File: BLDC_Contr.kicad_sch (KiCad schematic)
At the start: 100 parts, among them J1 XT60, J10 PH, J2 Conn_ARM_SWD_TagConnect_TC2030, J3 PH, J4 PH, J5 PH, J6 PH, J7 PH, J8 PIN, Q1 CSD18540Q5B, Q2 CSD18540Q5B, Q3 CSD18540Q5B, Q4 CSD18540Q5B, Q5 CSD18540Q5B, Q6 CSD18540Q5B, U1 STM32G431CBU6, U2 DRV8323RSRGZR, U3 AMS1117-3.3, Y1 Crystal_16Mhz

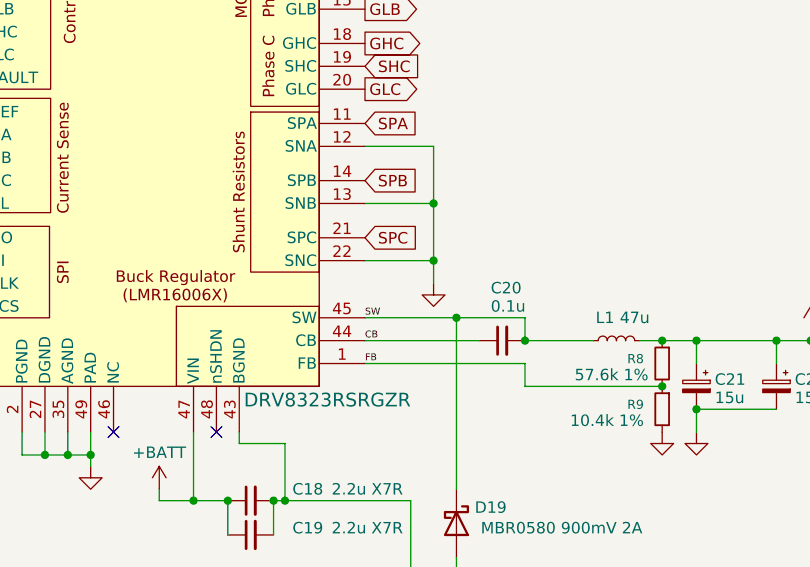
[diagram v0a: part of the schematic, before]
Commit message: wired every component, ground poured doing erc (not done yet)
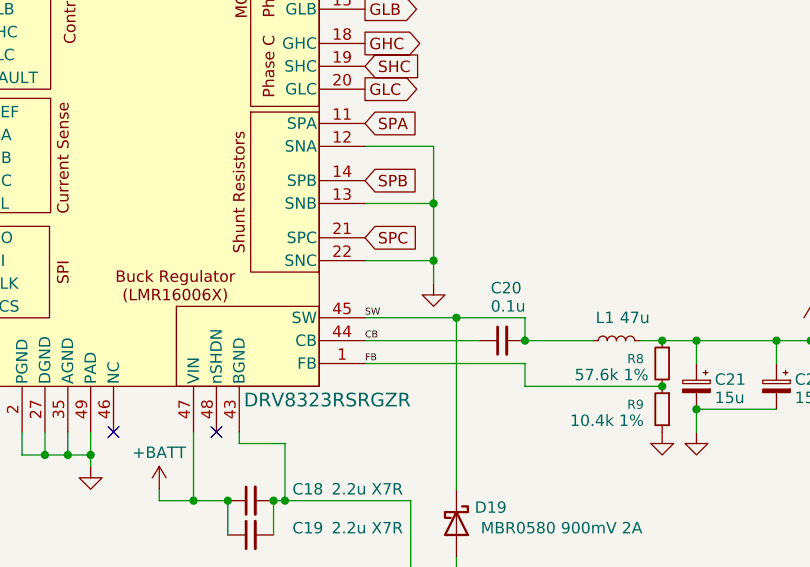
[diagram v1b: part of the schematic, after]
